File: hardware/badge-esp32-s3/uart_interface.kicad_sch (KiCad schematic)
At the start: 17 parts, among them Q1 SS8050 200-350, Q2 SS8050 200-350, U3 CP2102N-A02-GQFN28R

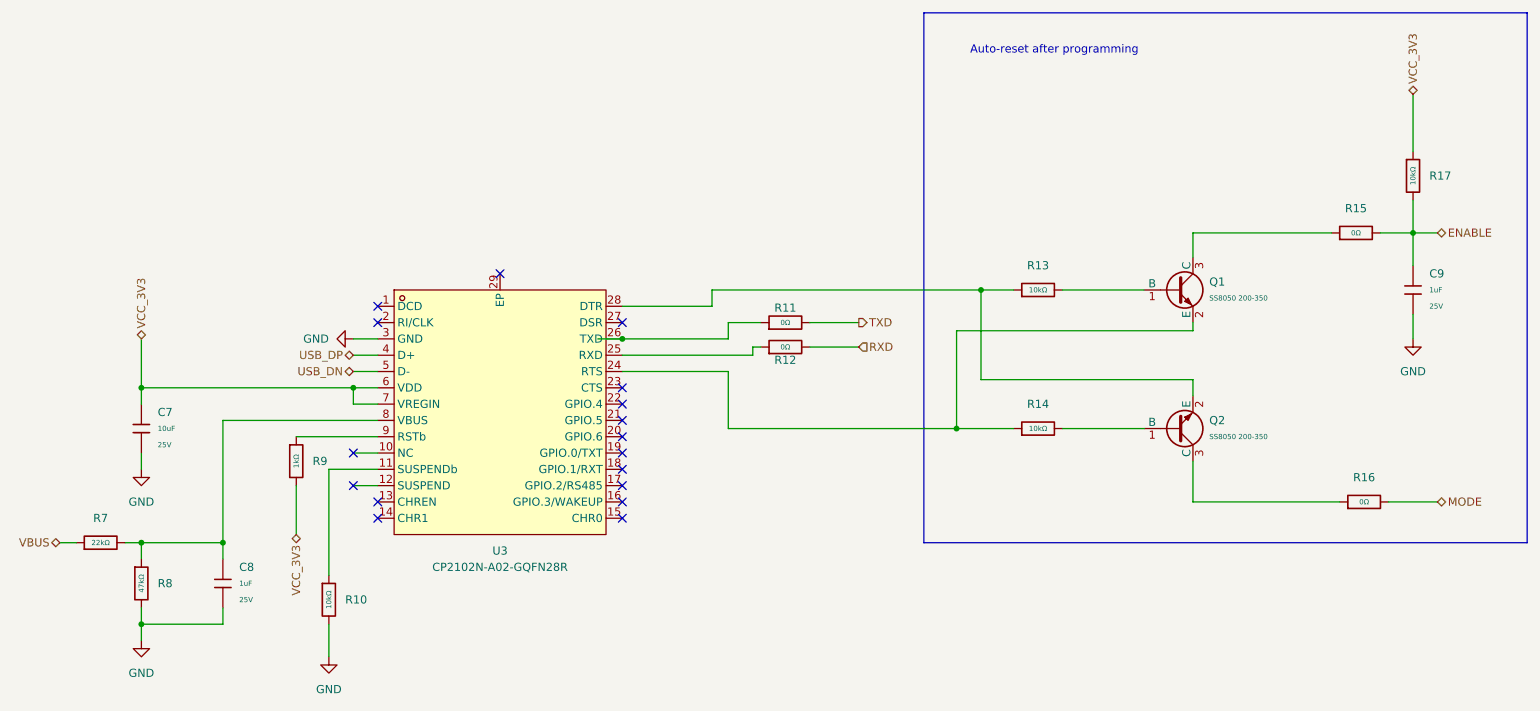
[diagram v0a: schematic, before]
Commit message: almost finished
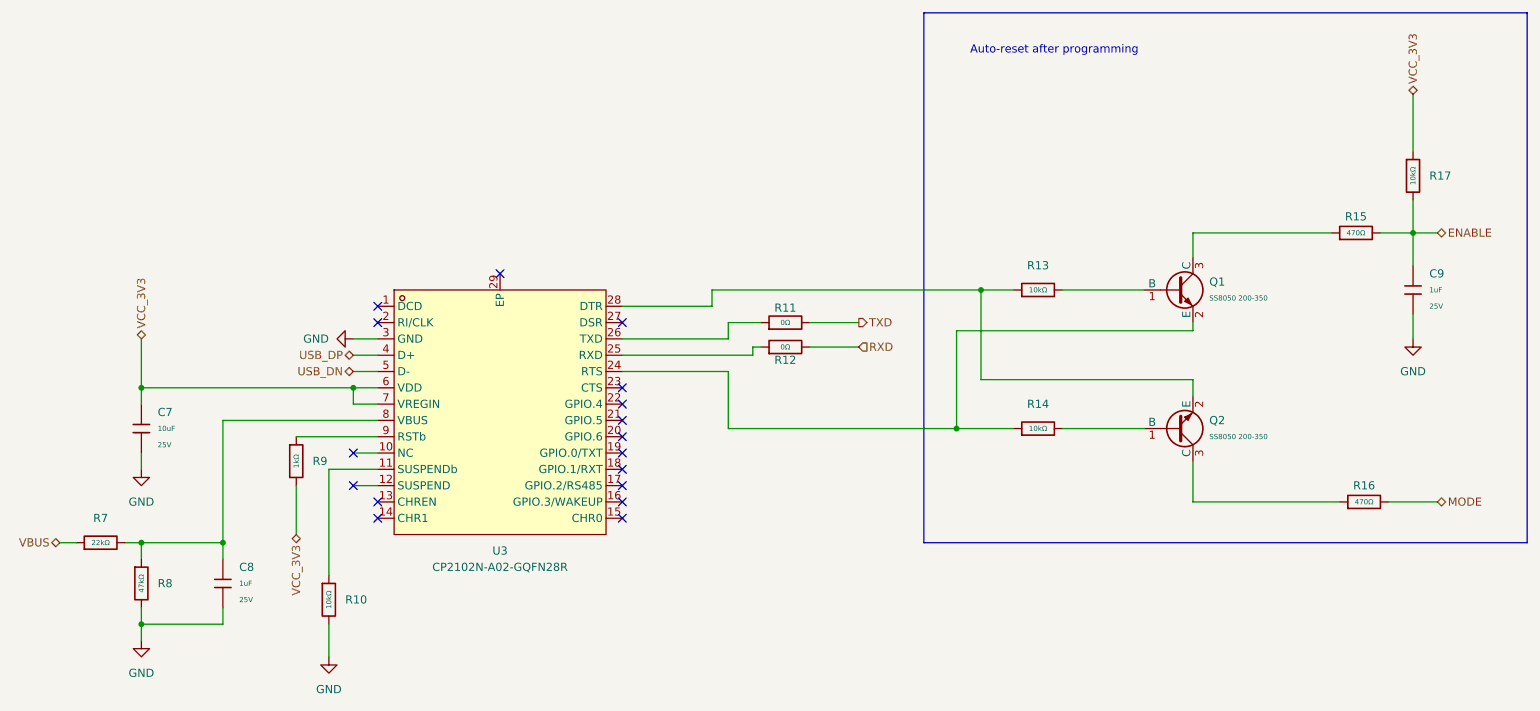
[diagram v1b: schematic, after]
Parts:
- removed R15, R16: 0Ω, PCM_JLCPCB:R_0402, symbol PCM_JLCPCB-Resistors:0402,0Ω
- added R15, R16: 470Ω, PCM_JLCPCB:R_0402, symbol PCM_JLCPCB-Resistors:0402,470Ω
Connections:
- net ENABLE: now also R15.2
- net MODE: now also R16.2
- net at Q1.3 (C): now also R15.1
- net at Q2.3 (C): now also R16.1
